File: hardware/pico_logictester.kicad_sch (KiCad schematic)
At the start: 18 parts

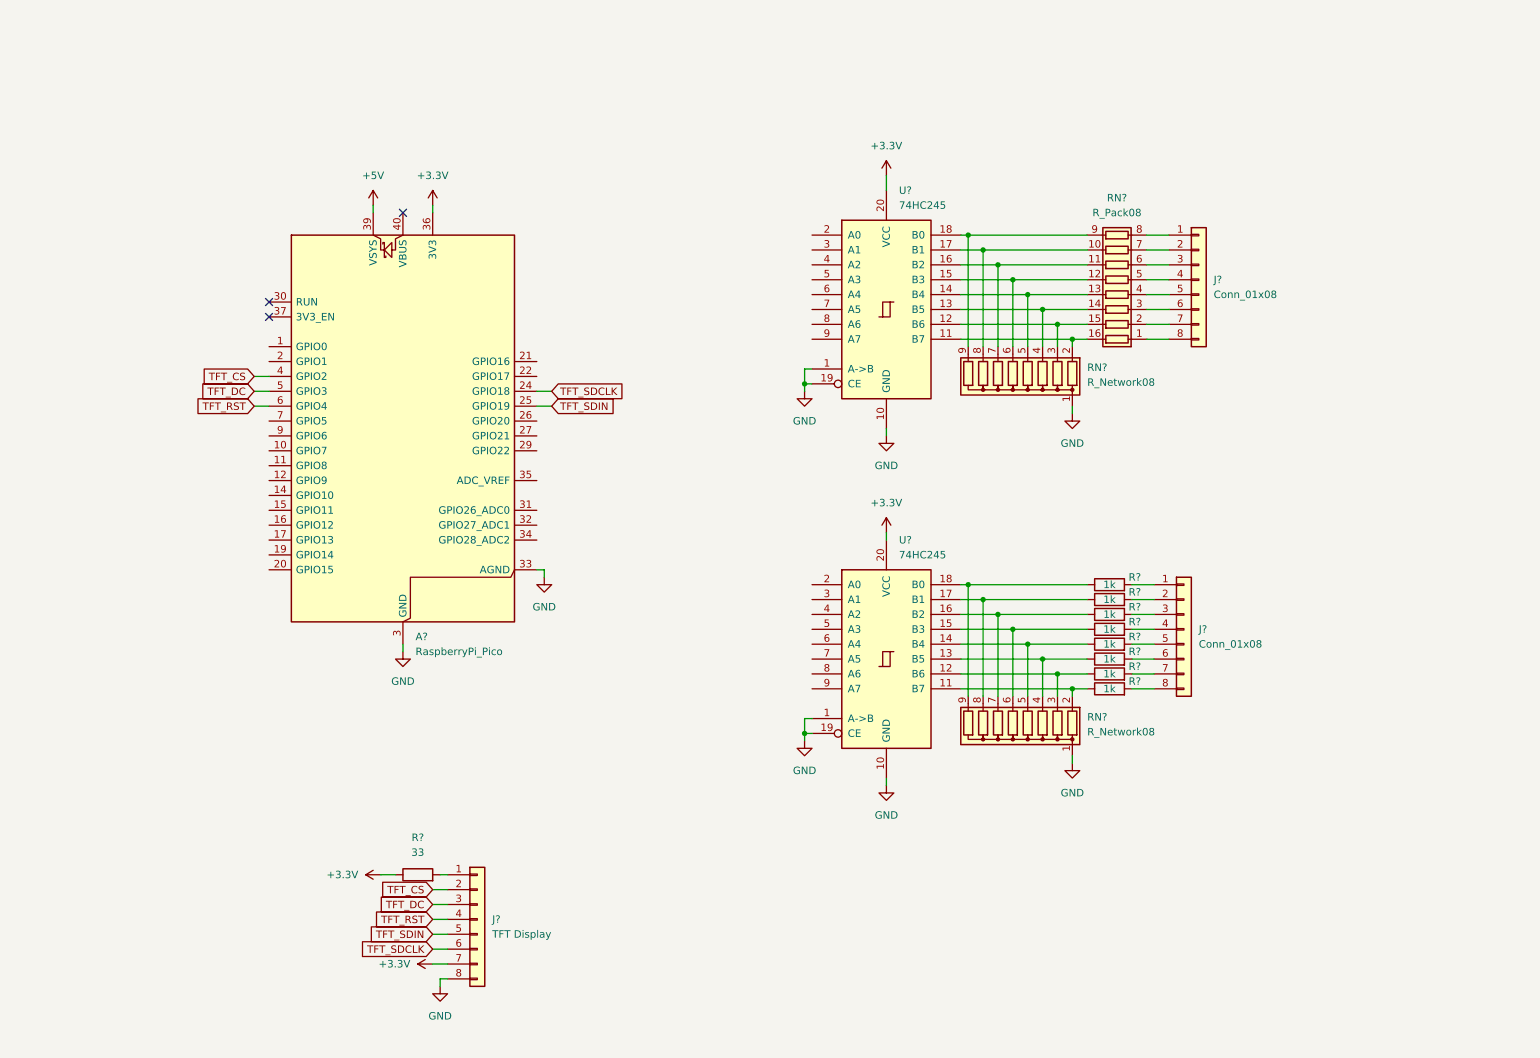
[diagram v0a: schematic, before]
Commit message: hardware: Alle baugruppen im schaltplan hinzugefügt.
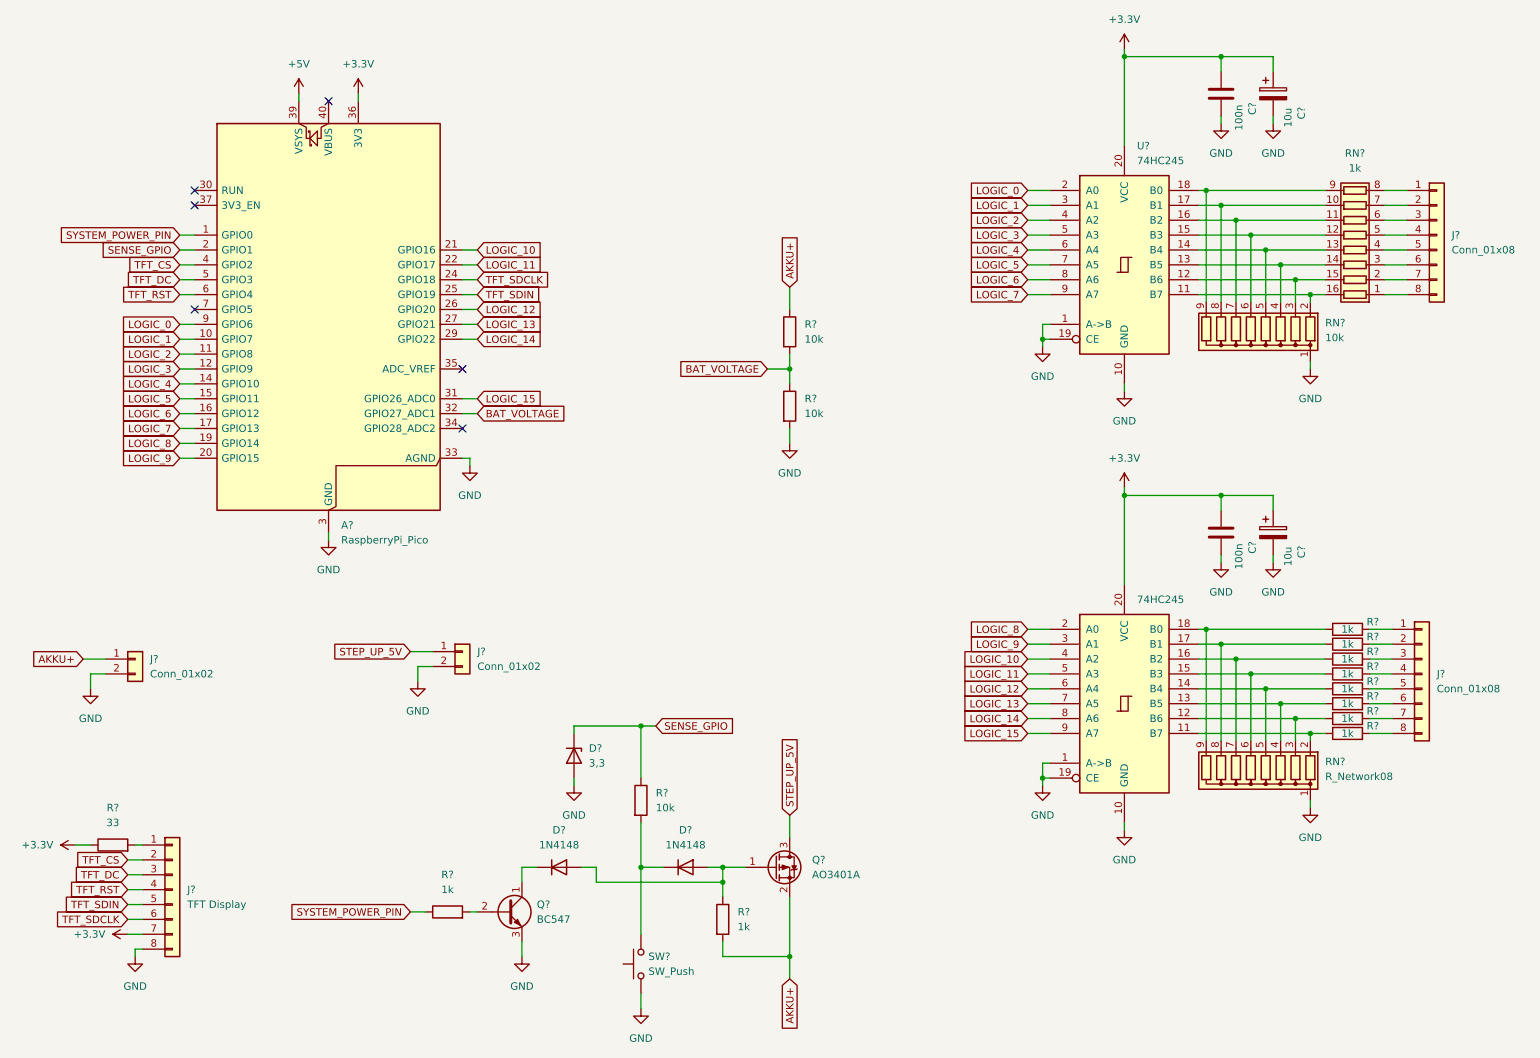
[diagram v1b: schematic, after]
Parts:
- added C? (x2): 100n, symbol Device:C
- added C? (x2): 10u, symbol Device:C_Polarized
- added D? (x2): 1N4148, Diode_THT:D_DO-35_SOD27_P7.62mm_Horizontal, symbol Diode:1N4148
- added D?: 3,3, symbol Device:D_Zener
- added J? (x2): Conn_01x02, symbol Connector_Generic:Conn_01x02
- added Q?: AO3401A, Package_TO_SOT_SMD:SOT-23, symbol Transistor_FET:AO3401A
- added Q?: BC547, Package_TO_SOT_THT:TO-92_Inline, symbol Transistor_BJT:BC547
- added R? (x3): 10k, symbol Device:R
- added R? (x2): 1k, symbol Device:R
- added SW?: SW_Push, symbol Switch:SW_Push
- RN?: value R_Pack08 -> 1k
- RN?: value R_Network08 -> 10k
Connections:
- net +3.3V: now also C?.1, C?.1, C?.1, C?.1
- net GND: now also C?.2, C?.2, C?.2, C?.2, D?.2 (A), J?.2 (Pin_2), J?.2 (Pin_2), Q?.3 (E), R?.2, SW?.1
- net SYSTEM_POWER_PIN: now reaches A?.1 (GPIO0)
- net SYSTEM_POWER_PIN: now also R?.1
- net LOGIC_1: now reaches A?.10 (GPIO7)
- net LOGIC_1: now also U?.3 (A1)
- net LOGIC_2: now reaches A?.11 (GPIO8)
- net LOGIC_2: now also U?.4 (A2)
- net LOGIC_3: now reaches A?.12 (GPIO9)
- net LOGIC_3: now also U?.5 (A3)
- net LOGIC_4: now reaches A?.14 (GPIO10)
- net LOGIC_4: now also U?.6 (A4)
- net LOGIC_5: now reaches A?.15 (GPIO11)
- net LOGIC_5: now also U?.7 (A5)
- net LOGIC_6: now reaches A?.16 (GPIO12)
- net LOGIC_6: now also U?.8 (A6)
- net LOGIC_7: now reaches A?.17 (GPIO13)
- net LOGIC_7: now also U?.9 (A7)
- net LOGIC_8: now reaches A?.19 (GPIO14)
- net LOGIC_8: now also U?.2 (A0)
- net SENSE_GPIO: now reaches A?.2 (GPIO1)
- net SENSE_GPIO: now also D?.1 (K), R?.1
- net LOGIC_9: now reaches A?.20 (GPIO15)
- net LOGIC_9: now also U?.3 (A1)
- net LOGIC_10: now reaches A?.21 (GPIO16)
- net LOGIC_10: now also U?.4 (A2)
- net LOGIC_11: now reaches A?.22 (GPIO17)
- net LOGIC_11: now also U?.5 (A3)
- net LOGIC_12: now reaches A?.26 (GPIO20)
- net LOGIC_12: now also U?.6 (A4)
- net LOGIC_13: now reaches A?.27 (GPIO21)
- net LOGIC_13: now also U?.7 (A5)
- net LOGIC_14: now reaches A?.29 (GPIO22)
- net LOGIC_14: now also U?.8 (A6)
- net LOGIC_15: now reaches A?.31 (GPIO26_ADC0)
- net LOGIC_15: now also U?.9 (A7)
- net BAT_VOLTAGE: now reaches A?.32 (GPIO27_ADC1)
- net BAT_VOLTAGE: now also R?.1, R?.2
- net LOGIC_0: now reaches A?.9 (GPIO6)
- net LOGIC_0: now also U?.2 (A0)
- new net: D?.1 (K), Q?.1 (C)
- new net: D?.2 (A), D?.2 (A), Q?.1 (G), R?.1
- new net: D?.1 (K), R?.2, SW?.2
- new net: Q?.2 (B), R?.2
- new net AKKU+: J?.1 (Pin_1), Q?.2 (S), R?.1, R?.2
- new net STEP_UP_5V: J?.1 (Pin_1), Q?.3 (D)
- no-connect marks 3 -> 6
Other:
- moved on the sheet: A?, J?, R?, RN?, U?
